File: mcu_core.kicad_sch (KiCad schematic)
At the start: 17 parts, among them U5 TMS5700714APGEQQ1R

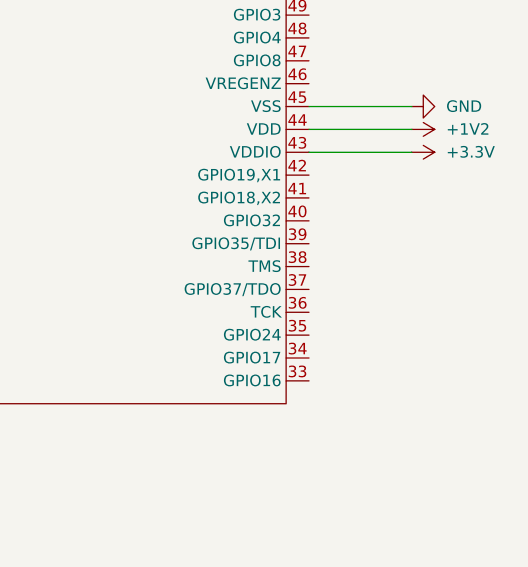
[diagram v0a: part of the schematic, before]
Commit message: #
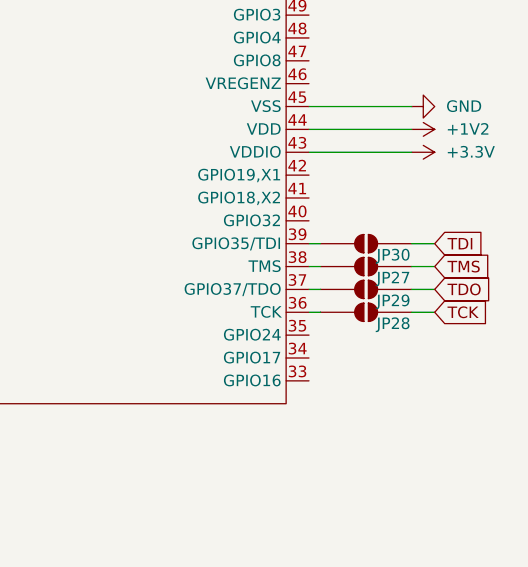
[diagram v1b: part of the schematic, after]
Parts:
- added JP27, JP28, JP29, JP30: SolderJumper_2_Open, symbol Jumper:SolderJumper_2_Open
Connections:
- net TCK: now also JP28.1 (A)
- net TDI: now also JP30.1 (A)
- net TDO: now also JP29.1 (A)
- net TMS: now also JP27.2 (B)
- net at U11.36 (TCK): now also JP28.2 (B)
- net at U11.37 (GPIO37/TDO): now also JP29.2 (B)
- net at U11.38 (TMS): now also JP27.1 (A)
- net at U11.39 (GPIO35/TDI): now also JP30.2 (B)

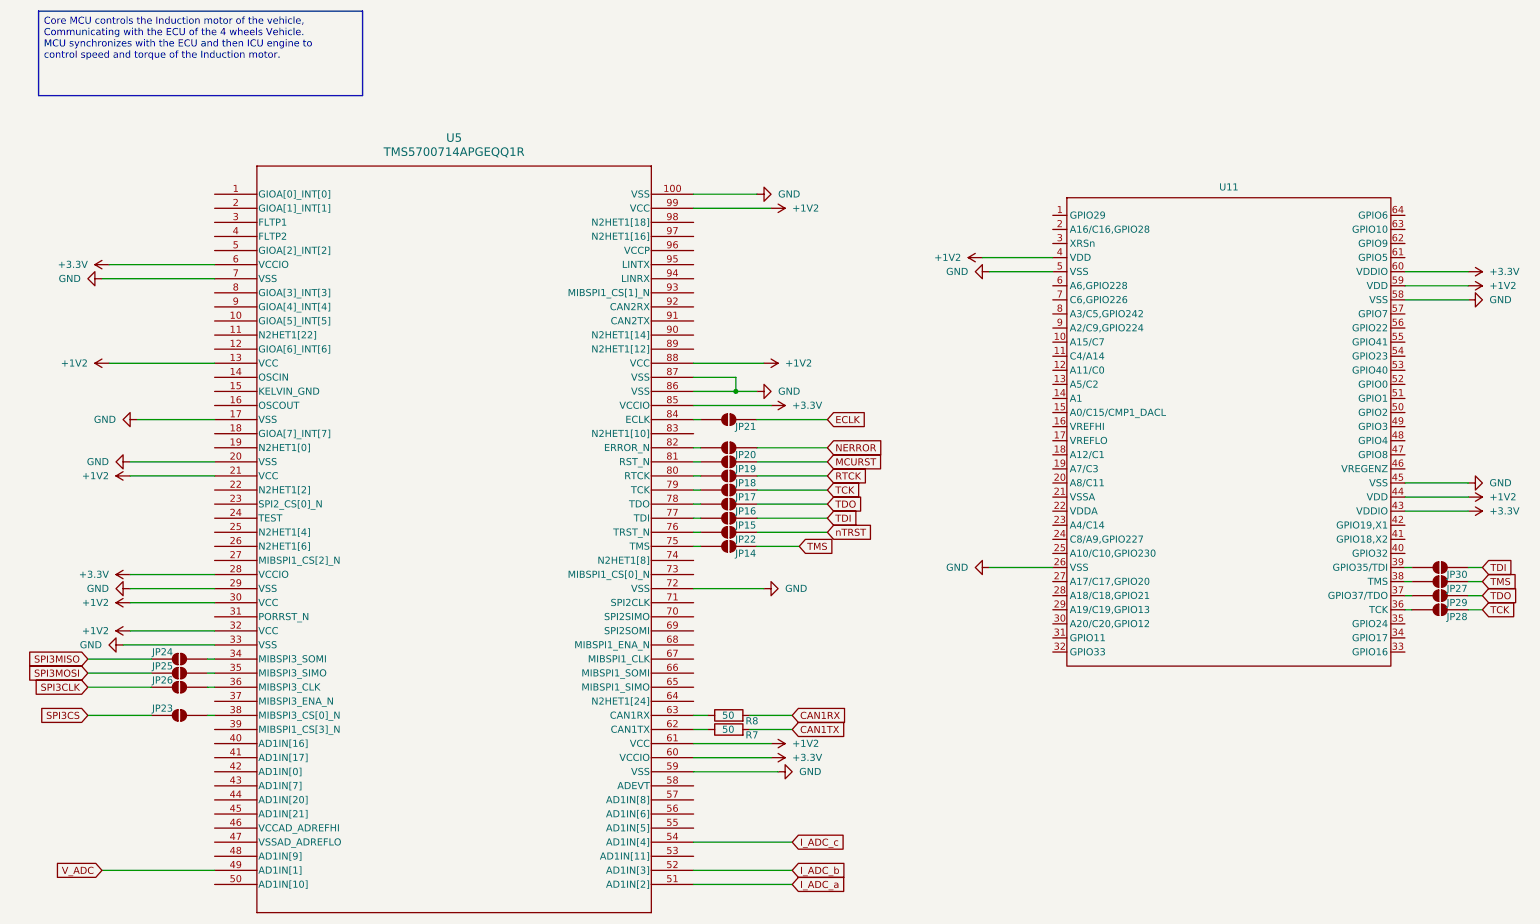
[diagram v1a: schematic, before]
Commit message: #
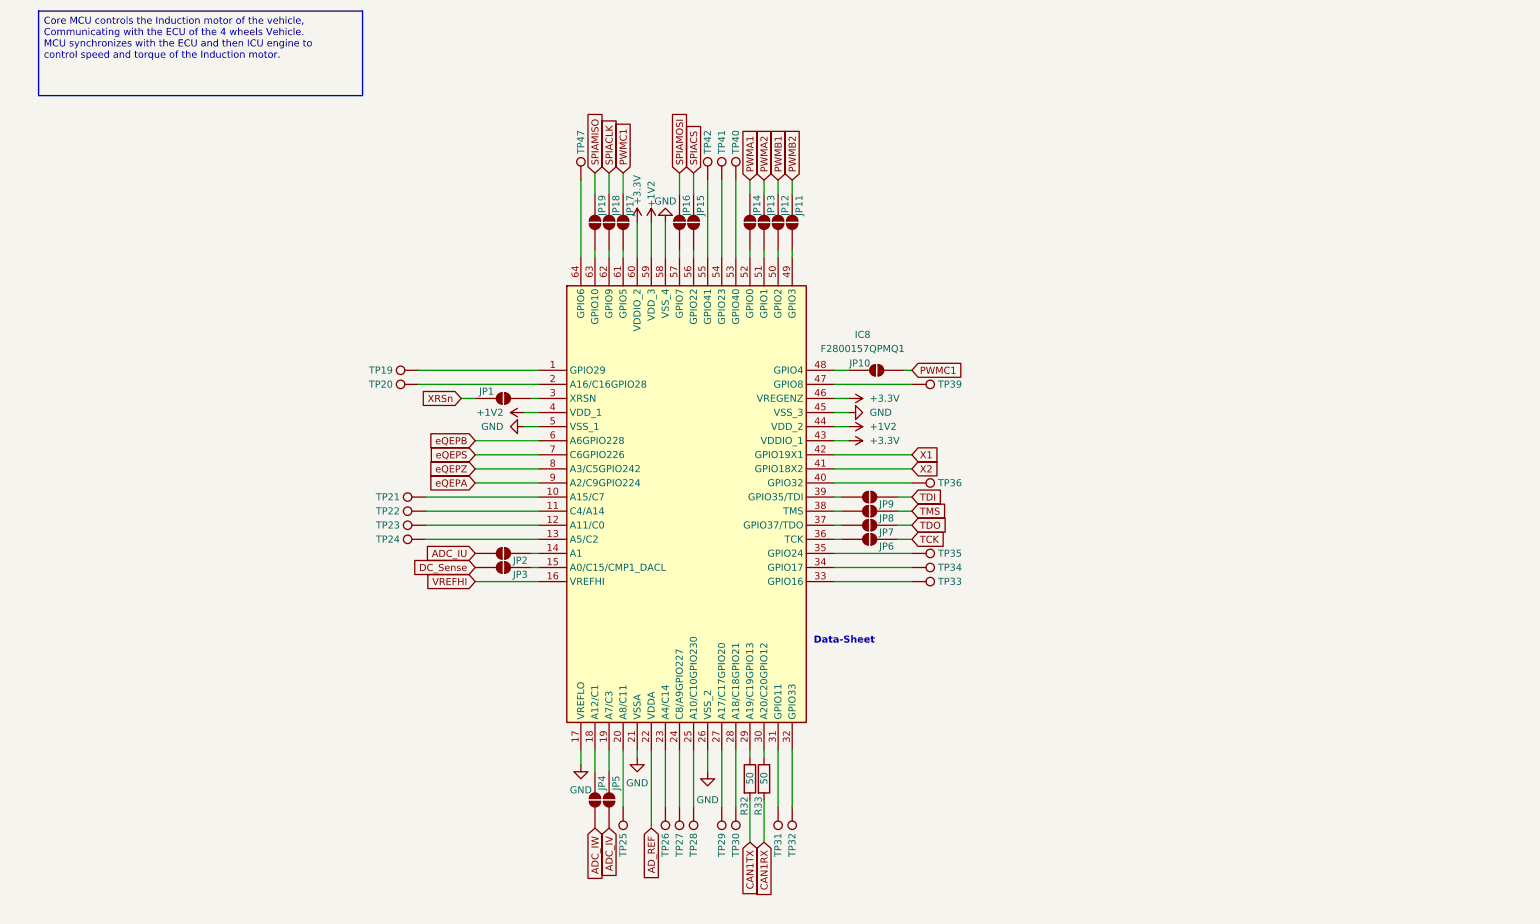
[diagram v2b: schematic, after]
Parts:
- removed JP20, JP21, JP22, JP23, JP24, JP25, JP26, JP27, JP28, JP29, JP30: SolderJumper_2_Open, symbol Jumper:SolderJumper_2_Open
- removed R7, R8: 50, symbol Device:R
- removed U11: (no value), symbol Library:TMS320F2800157-Q1
- removed U5: TMS5700714APGEQQ1R, PZ0100A_N_TEX, symbol TMS5700714APGEQQ1R:TMS5700714APGEQQ1R
- added IC8: F2800157QPMQ1, Footprint:QFP50P1200X1200X160-64N, symbol F2800157QPMQ1:F2800157QPMQ1
- added JP1, JP10, JP11, JP12, JP13, JP2, JP3, JP4, JP5, JP6, JP7, JP8, JP9: SolderJumper_2_Open, symbol Jumper:SolderJumper_2_Open
- added R32, R33: 50, symbol Device:R
- added TP19, TP20, TP21, TP22, TP23, TP24, TP25, TP26, TP27, TP28, TP29, TP30, TP31, TP32, TP33, TP34, TP35, TP36, TP39, TP40, TP41, TP42, TP47: TestPoint, symbol Connector:TestPoint
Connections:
- net +1V2: now also IC8.4 (VDD_1), IC8.44 (VDD_2), IC8.59 (VDD_3)
- net +3.3V: now also IC8.43 (VDDIO_1), IC8.46 (VREGENZ), IC8.60 (VDDIO_2)
- net CAN1RX: now also R33.2
- net CAN1TX: now also R32.2
- net GND: now also IC8.17 (VREFLO), IC8.21 (VSSA), IC8.26 (VSS_2), IC8.45 (VSS_3), IC8.5 (VSS_1), IC8.58 (VSS_4)
- net TCK: now also JP6.1 (A); no longer JP17.1 (A)
- net TDI: now also JP9.1 (A); no longer JP15.1 (A)
- net TDO: now also JP7.1 (A); no longer JP16.1 (A)
- net TMS: now also JP8.2 (B); no longer JP14.2 (B)
- net at JP15.2 (B): now also IC8.56 (GPIO22)
- net at JP17.2 (B): now also IC8.61 (GPIO5)
- net PWMA1: now reaches JP14.1 (A)
- net at JP16.2 (B): now also IC8.57 (GPIO7)
- net at JP18.2 (B): now also IC8.62 (GPIO9)
- net at JP19.2 (B): now also IC8.63 (GPIO10)
- net MCURST renamed SPIAMISO
- net RTCK renamed SPIACLK
- new net: IC8.49 (GPIO3), JP11.2 (B)
- new net: IC8.11 (C4/A14), TP22.1
- new net: IC8.20 (A8/C11), TP25.1
- new net: IC8.52 (GPIO0), JP14.2 (B)
- new net: IC8.54 (GPIO23), TP41.1
- new net: IC8.47 (GPIO8), TP39.1
- new net: IC8.27 (A17/C17GPIO20), TP29.1
- new net: IC8.53 (GPIO40), TP40.1
- new net: IC8.40 (GPIO32), TP36.1
- new net: IC8.1 (GPIO29), TP19.1
- new net: IC8.10 (A15/C7), TP21.1
- new net: IC8.12 (A11/C0), TP23.1
- new net: IC8.13 (A5/C2), TP24.1
- new net: IC8.14 (A1), JP2.1 (A)
- new net: IC8.15 (A0/C15/CMP1_DACL), JP3.1 (A)
- new net: IC8.18 (A12/C1), JP4.1 (A)
- new net: IC8.19 (A7/C3), JP5.1 (A)
- new net: IC8.2 (A16/C16GPIO28), TP20.1
- new net: IC8.23 (A4/C14), TP26.1
- new net: IC8.24 (C8/A9GPIO227), TP27.1
- new net: IC8.25 (A10/C10GPIO230), TP28.1
- new net: IC8.28 (A18/C18GPIO21), TP30.1
- new net: IC8.29 (A19/C19GPIO13), R32.1
- new net: IC8.3 (XRSN), JP1.2 (B)
- new net: IC8.30 (A20/C20GPIO12), R33.1
- new net: IC8.31 (GPIO11), TP31.1
- new net: IC8.32 (GPIO33), TP32.1
- new net: IC8.33 (GPIO16), TP33.1
- new net: IC8.34 (GPIO17), TP34.1
- new net: IC8.35 (GPIO24), TP35.1
- new net: IC8.36 (TCK), JP6.2 (B)
- new net: IC8.37 (GPIO37/TDO), JP7.2 (B)
- new net: IC8.38 (TMS), JP8.1 (A)
- new net: IC8.39 (GPIO35/TDI), JP9.2 (B)
- new net: IC8.48 (GPIO4), JP10.1 (A)
- new net: IC8.50 (GPIO2), JP12.2 (B)
- new net: IC8.51 (GPIO1), JP13.2 (B)
- new net: IC8.55 (GPIO41), TP42.1
- new net: IC8.64 (GPIO6), TP47.1
- new net ADC_IU: JP2.2 (B)
- new net ADC_IV: JP5.2 (B)
- new net ADC_IW: JP4.2 (B)
- new net AD_REF: IC8.22 (VDDA)
- new net DC_Sense: JP3.2 (B)
- new net PWMA2: JP13.1 (A)
- new net PWMB1: JP12.1 (A)
- new net PWMB2: JP11.1 (A)
- new net PWMC1: JP10.2 (B), JP17.1 (A)
- new net SPIACS: JP15.1 (A)
- new net SPIAMOSI: JP16.1 (A)
- new net VREFHI: IC8.16 (VREFHI)
- new net X1: IC8.42 (GPIO19X1)
- new net X2: IC8.41 (GPIO18X2)
- new net XRSn: JP1.1 (A)
- new net eQEPA: IC8.9 (A2/C9GPIO224)
- new net eQEPB: IC8.6 (A6GPIO228)
- new net eQEPS: IC8.7 (C6GPIO226)
- new net eQEPZ: IC8.8 (A3/C5GPIO242)
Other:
- note added: "Data-Sheet"
